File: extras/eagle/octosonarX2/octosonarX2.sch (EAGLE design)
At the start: 45 parts, among them IC1 74HC125D, IC2 74HC125D, IC3 74HC125D, IC4 74HC125D, IC5 PCF8575C

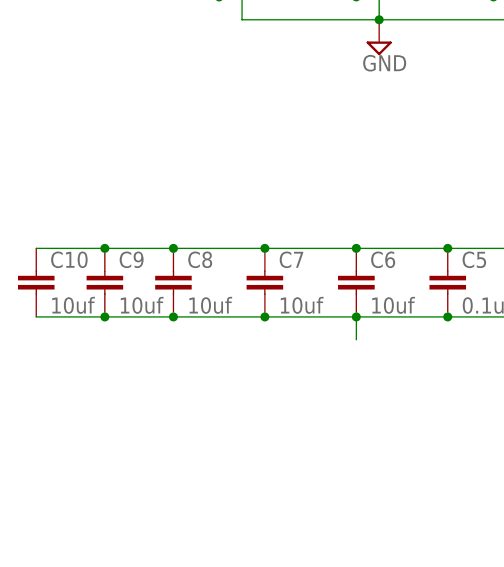
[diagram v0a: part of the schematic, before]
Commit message: 1.2.0 eagle files and examples updated
Eagle files updated for OctoSonarX2 and Trimounts to reflect modifications between prototype and production.

OctoSonarX2 - tweaked bypass caps. Rerouted 5V with wider traces.
Examples - tidies up with serial only tests and separate LCD tests.
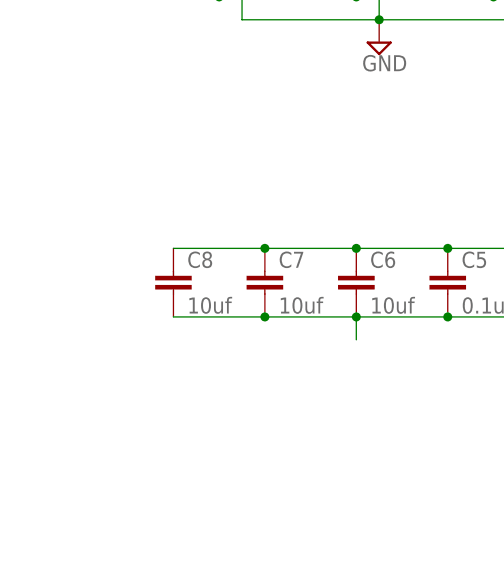
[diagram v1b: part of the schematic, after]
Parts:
- removed C10, C9: 10uf, resistor:C-EUC0603
- C7, C8: device resistor:C-EUC0603 -> resistor:C-EUC0805
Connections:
- net GND: no longer C10.2, C9.2
- net VCC: no longer C10.1, C9.1
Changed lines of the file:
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@@
 <part name="C5" library="resistor" library_urn="urn:adsk.eagle:library:348" deviceset="C-EU" device="C0603" value="0.1uf"/>
 <part name="C6" library="resistor" library_urn="urn:adsk.eagle:library:348" deviceset="C-EU" device="C0603" value="10uf"/>
-<part name="C7" library="resistor" library_urn="urn:adsk.eagle:library:348" deviceset="C-EU" device="C0603" value="10uf"/>
-<part name="C8" library="resistor" library_urn="urn:adsk.eagle:library:348" deviceset="C-EU" device="C0603" value="10uf"/>
+<part name="C7" library="resistor" library_urn="urn:adsk.eagle:library:348" deviceset="C-EU" device="C0805" value="10uf"/>
+<part name="C8" library="resistor" library_urn="urn:adsk.eagle:library:348" deviceset="C-EU" device="C0805" value="10uf"/>
 <part name="J3" library="SparkFun-Connectors" deviceset="CONN_02" device=""/>
 <part name="J4" library="SparkFun-Connectors" deviceset="CONN_02" device=""/>
@@
 <part name="SUPPLY41" library="supply2" deviceset="+5V" device=""/>
 <part name="SUPPLY42" library="supply2" deviceset="GND" device=""/>
-<part name="C9" library="resistor" library_urn="urn:adsk.eagle:library:348" deviceset="C-EU" device="C0603" value="10uf"/>
-<part name="C10" library="resistor" library_urn="urn:adsk.eagle:library:348" deviceset="C-EU" device="C0603" value="10uf"/>
 <part name="LOGO1" library="SparkFun-Aesthetics" deviceset="OSHW-LOGO" device="L"/>
 </parts>
@@
 <instance part="SUPPLY41" gate="+5V" x="-124.46" y="12.7"/>
 <instance part="SUPPLY42" gate="GND" x="-96.52" y="-10.16"/>
-<instance part="C9" gate="G$1" x="-127" y="-35.56"/>
-<instance part="C10" gate="G$1" x="-134.62" y="-35.56"/>
 <instance part="LOGO1" gate="G$1" x="-43.18" y="-60.96"/>
 </instances>
@@
 <wire x1="-109.22" y1="-40.64" x2="-119.38" y2="-40.64" width="0.1524" layer="91"/>
 <junction x="-109.22" y="-40.64"/>
-<pinref part="C10" gate="G$1" pin="2"/>
-<pinref part="C9" gate="G$1" pin="2"/>
-<wire x1="-134.62" y1="-40.64" x2="-127" y2="-40.64" width="0.1524" layer="91"/>
-<wire x1="-127" y1="-40.64" x2="-119.38" y2="-40.64" width="0.1524" layer="91"/>
-<junction x="-127" y="-40.64"/>
-<junction x="-119.38" y="-40.64"/>
 </segment>
 <segment>
@@
 <wire x1="-109.22" y1="-33.02" x2="-119.38" y2="-33.02" width="0.1524" layer="91"/>
 <junction x="-109.22" y="-33.02"/>
-<pinref part="C10" gate="G$1" pin="1"/>
-<pinref part="C9" gate="G$1" pin="1"/>
-<wire x1="-134.62" y1="-33.02" x2="-127" y2="-33.02" width="0.1524" layer="91"/>
-<wire x1="-127" y1="-33.02" x2="-119.38" y2="-33.02" width="0.1524" layer="91"/>
-<junction x="-127" y="-33.02"/>
-<junction x="-119.38" y="-33.02"/>
-</segment>
-<segment>
+</segment>
+<segment>

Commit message: Revert "Updates to X2 test and trimount bracket"
This reverts commit f0c77c11ce1398fcc169d7c2890869ee86536cf6.
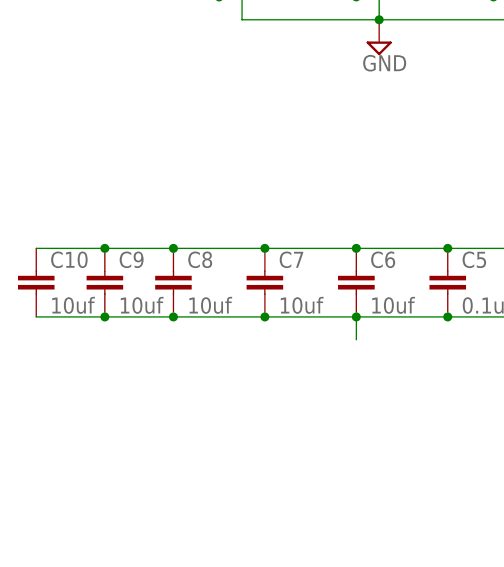
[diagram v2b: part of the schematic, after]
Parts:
- added C10, C9: 10uf, resistor:C-EUC0603
- C7, C8: device resistor:C-EUC0805 -> resistor:C-EUC0603
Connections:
- net GND: now also C10.2, C9.2
- net VCC: now also C10.1, C9.1
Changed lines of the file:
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@@
 <part name="C5" library="resistor" library_urn="urn:adsk.eagle:library:348" deviceset="C-EU" device="C0603" value="0.1uf"/>
 <part name="C6" library="resistor" library_urn="urn:adsk.eagle:library:348" deviceset="C-EU" device="C0603" value="10uf"/>
-<part name="C7" library="resistor" library_urn="urn:adsk.eagle:library:348" deviceset="C-EU" device="C0805" value="10uf"/>
-<part name="C8" library="resistor" library_urn="urn:adsk.eagle:library:348" deviceset="C-EU" device="C0805" value="10uf"/>
+<part name="C7" library="resistor" library_urn="urn:adsk.eagle:library:348" deviceset="C-EU" device="C0603" value="10uf"/>
+<part name="C8" library="resistor" library_urn="urn:adsk.eagle:library:348" deviceset="C-EU" device="C0603" value="10uf"/>
 <part name="J3" library="SparkFun-Connectors" deviceset="CONN_02" device=""/>
 <part name="J4" library="SparkFun-Connectors" deviceset="CONN_02" device=""/>
@@
 <part name="SUPPLY41" library="supply2" deviceset="+5V" device=""/>
 <part name="SUPPLY42" library="supply2" deviceset="GND" device=""/>
+<part name="C9" library="resistor" library_urn="urn:adsk.eagle:library:348" deviceset="C-EU" device="C0603" value="10uf"/>
+<part name="C10" library="resistor" library_urn="urn:adsk.eagle:library:348" deviceset="C-EU" device="C0603" value="10uf"/>
 <part name="LOGO1" library="SparkFun-Aesthetics" deviceset="OSHW-LOGO" device="L"/>
 </parts>
@@
 <instance part="SUPPLY41" gate="+5V" x="-124.46" y="12.7"/>
 <instance part="SUPPLY42" gate="GND" x="-96.52" y="-10.16"/>
+<instance part="C9" gate="G$1" x="-127" y="-35.56"/>
+<instance part="C10" gate="G$1" x="-134.62" y="-35.56"/>
 <instance part="LOGO1" gate="G$1" x="-43.18" y="-60.96"/>
 </instances>
@@
 <wire x1="-109.22" y1="-40.64" x2="-119.38" y2="-40.64" width="0.1524" layer="91"/>
 <junction x="-109.22" y="-40.64"/>
+<pinref part="C10" gate="G$1" pin="2"/>
+<pinref part="C9" gate="G$1" pin="2"/>
+<wire x1="-134.62" y1="-40.64" x2="-127" y2="-40.64" width="0.1524" layer="91"/>
+<wire x1="-127" y1="-40.64" x2="-119.38" y2="-40.64" width="0.1524" layer="91"/>
+<junction x="-127" y="-40.64"/>
+<junction x="-119.38" y="-40.64"/>
 </segment>
 <segment>
@@
 <wire x1="-109.22" y1="-33.02" x2="-119.38" y2="-33.02" width="0.1524" layer="91"/>
 <junction x="-109.22" y="-33.02"/>
-</segment>
-<segment>
+<pinref part="C10" gate="G$1" pin="1"/>
+<pinref part="C9" gate="G$1" pin="1"/>
+<wire x1="-134.62" y1="-33.02" x2="-127" y2="-33.02" width="0.1524" layer="91"/>
+<wire x1="-127" y1="-33.02" x2="-119.38" y2="-33.02" width="0.1524" layer="91"/>
+<junction x="-127" y="-33.02"/>
+<junction x="-119.38" y="-33.02"/>
+</segment>
+<segment>
